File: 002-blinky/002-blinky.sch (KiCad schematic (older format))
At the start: 1 part

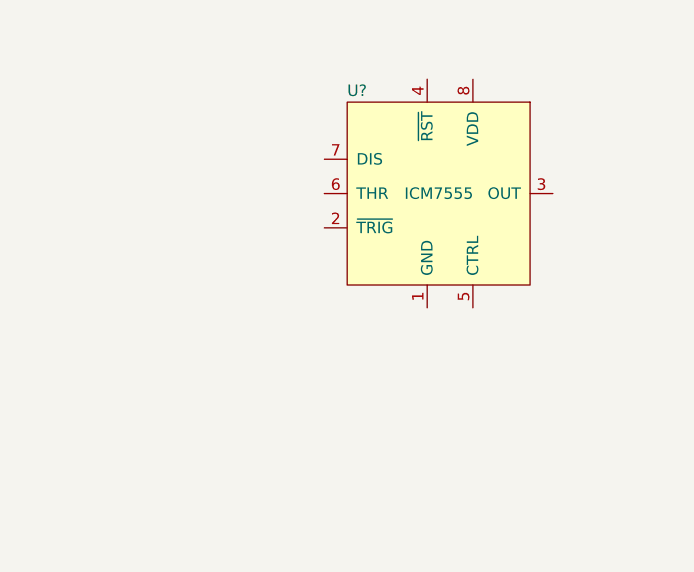
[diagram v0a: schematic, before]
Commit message: 002 schematic + 1bitsy files
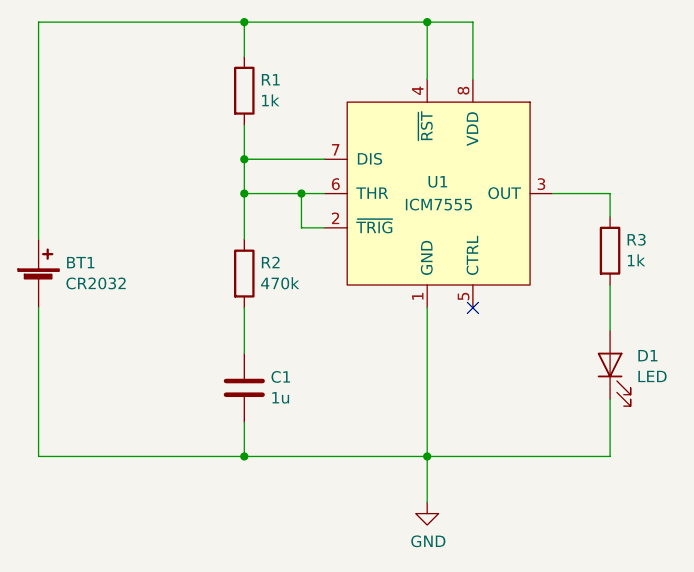
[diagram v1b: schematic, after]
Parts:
- removed U?: ICM7555, symbol 002-blinky:ICM7555
- added BT1: CR2032, symbol 002-blinky:CR2032
- added C1: 1u, symbol Device:C
- added D1: LED, symbol Device:LED
- added R1, R3: 1k, symbol Device:R
- added R2: 470k, symbol Device:R
- added U1: ICM7555, symbol 002-blinky:ICM7555
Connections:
- new net: BT1.1 (+), R1.1, U1.4 (~RST), U1.8 (VDD)
- new net: R1.2, R2.1, U1.2 (~TRIG), U1.6 (THR), U1.7 (DIS)
- new net: C1.1, R2.2
- new net: R3.1, U1.3 (OUT)
- new net: D1.2 (A), R3.2
- new net GND: BT1.2 (-), C1.2, D1.1 (K), U1.1 (GND)
- no-connect marks 0 -> 1
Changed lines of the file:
@@
 $EndDescr
 $Comp
-L 002-blinky:ICM7555 U?
-U 1 1 5E28BC5F
+L Device:R R1
+U 1 1 5E389841
+P 6350 4350
+F 0 "R1" H 6420 4396 50  0000 L CNN
+F 1 "1k" H 6420 4305 50  0000 L CNN
+F 2 "" V 6280 4350 50  0001 C CNN
+F 3 "~" H 6350 4350 50  0001 C CNN
+	1    6350 4350
+	1    0    0    -1
+$EndComp
+$Comp
+L Device:R R2
+U 1 1 5E389C17
+P 6350 5150
+F 0 "R2" H 6420 5196 50  0000 L CNN
+F 1 "470k" H 6420 5105 50  0000 L CNN
+F 2 "" V 6280 5150 50  0001 C CNN
+F 3 "~" H 6350 5150 50  0001 C CNN
+	1    6350 5150
+	1    0    0    -1
+$EndComp
+$Comp
+L Device:R R3
+U 1 1 5E389E08
+P 7950 5050
+F 0 "R3" H 8020 5096 50  0000 L CNN
+F 1 "1k" H 8020 5005 50  0000 L CNN
+F 2 "" V 7880 5050 50  0001 C CNN
+F 3 "~" H 7950 5050 50  0001 C CNN
+	1    7950 5050
+	1    0    0    -1
+$EndComp
+$Comp
+L Device:C C1
+U 1 1 5E38A4CC
+P 6350 5650
+F 0 "C1" H 6465 5696 50  0000 L CNN
+F 1 "1u" H 6465 5605 50  0000 L CNN
+F 2 "" H 6388 5500 50  0001 C CNN
+F 3 "~" H 6350 5650 50  0001 C CNN
+	1    6350 5650
+	1    0    0    -1
+$EndComp
+$Comp
+L Device:LED D1
+U 1 1 5E38A79B
+P 7950 5550
+F 0 "D1" V 7989 5433 50  0000 R CNN
+F 1 "LED" V 7898 5433 50  0000 R CNN
+F 2 "" H 7950 5550 50  0001 C CNN
+F 3 "~" H 7950 5550 50  0001 C CNN
+	1    7950 5550
+	0    -1   -1   0
+$EndComp
+Wire Wire Line
+	5450 5000 5450 4050
+Wire Wire Line
+	7350 4050 7350 4300
+Wire Wire Line
+	7150 4300 7150 4050
+Connection ~ 7150 4050
+Wire Wire Line
+	7150 4050 7350 4050
+Wire Wire Line
+	6350 4650 6350 4800
+Wire Wire Line
+	5450 4050 6350 4050
+Wire Wire Line
+	6700 4650 6350 4650
+Wire Wire Line
+	6350 4650 6350 4500
+Connection ~ 6350 4650
+Wire Wire Line
+	6350 4200 6350 4050
+Connection ~ 6350 4050
+Wire Wire Line
+	6350 4050 7150 4050
+Wire Wire Line
+	6700 4800 6600 4800
+Wire Wire Line
+	6600 4800 6600 4950
+Wire Wire Line
+	6600 4950 6700 4950
+Wire Wire Line
+	6600 4800 6350 4800
+Connection ~ 6600 4800
+Wire Wire Line
+	6350 5000 6350 4800
+Connection ~ 6350 4800
+Wire Wire Line
+	6350 5500 6350 5300
+Wire Wire Line
+	6350 5800 6350 5950
+Wire Wire Line
+	6350 5950 5450 5950
+Wire Wire Line
+	5450 5950 5450 5300
+Wire Wire Line
+	7150 5300 7150 5950
+Wire Wire Line
+	7150 5950 6350 5950
+Connection ~ 6350 5950
+$Comp
+L power:GND #PWR01
+U 1 1 5E392027
+P 7150 6150
+F 0 "#PWR01" H 7150 5900 50  0001 C CNN
+F 1 "GND" H 7155 5977 50  0000 C CNN
+F 2 "" H 7150 6150 50  0001 C CNN
+F 3 "" H 7150 6150 50  0001 C CNN
+	1    7150 6150
+	1    0    0    -1
+$EndComp
+Wire Wire Line
+	7150 6150 7150 5950
+Connection ~ 7150 5950
+Wire Wire Line
+	7700 4800 7950 4800
+Wire Wire Line
+	7950 4800 7950 4900
+Wire Wire Line
+	7950 5950 7150 5950
+Wire Wire Line
+	7950 5200 7950 5400
+Wire Wire Line
+	7950 5700 7950 5950
+NoConn ~ 7350 5300
+$Comp
+L 002-blinky:ICM7555 U1
+U 1 1 5E39F071
 P 7250 4800
-F 0 "U?" H 6800 5250 50  0000 L CNN
-F 1 "ICM7555" H 7050 4800 50  0000 L CNN
+F 0 "U1" H 7150 4850 50  0000 L CNN
+F 1 "ICM7555" H 7050 4750 50  0000 L CNN
 F 2 "" H 7150 5100 50  0001 C CNN
 F 3 "" H 7150 5100 50  0001 C CNN
@@
 	1    0    0    -1
 $EndComp
+$Comp
+L 002-blinky:CR2032 BT1
+U 1 1 5E38A2FB
+P 5450 5200
+F 0 "BT1" H 5568 5296 50  0000 L CNN
+F 1 "CR2032" H 5568 5205 50  0000 L CNN
+F 2 "" V 5450 5260 50  0001 C CNN
+F 3 "~" V 5450 5260 50  0001 C CNN
+	1    5450 5200
+	1    0    0    -1
+$EndComp
